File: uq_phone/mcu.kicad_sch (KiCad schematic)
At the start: 22 parts, among them J5 FTSH-105-XX-X-DV, J6 Conn_ARM_SWD_TagConnect_TC2030, U5 TXB0108RGYR, U6 TXB0108RGYR, U7 STM32H730VBTx

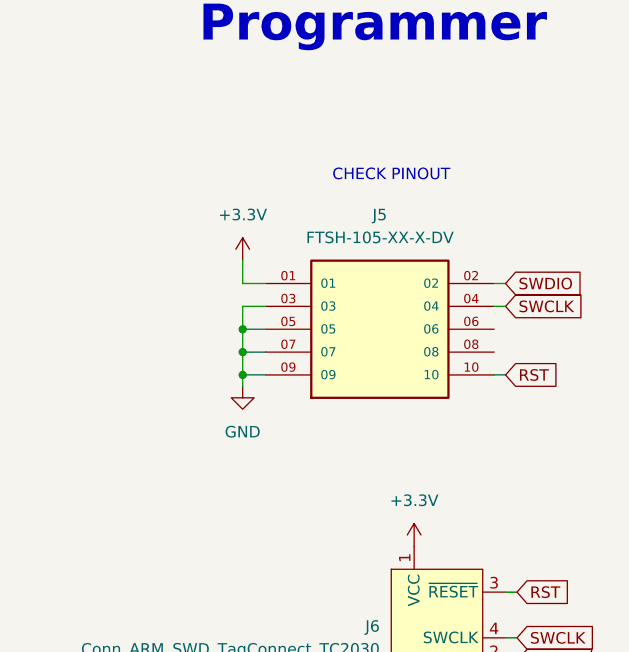
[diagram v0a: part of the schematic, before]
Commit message: Update routing
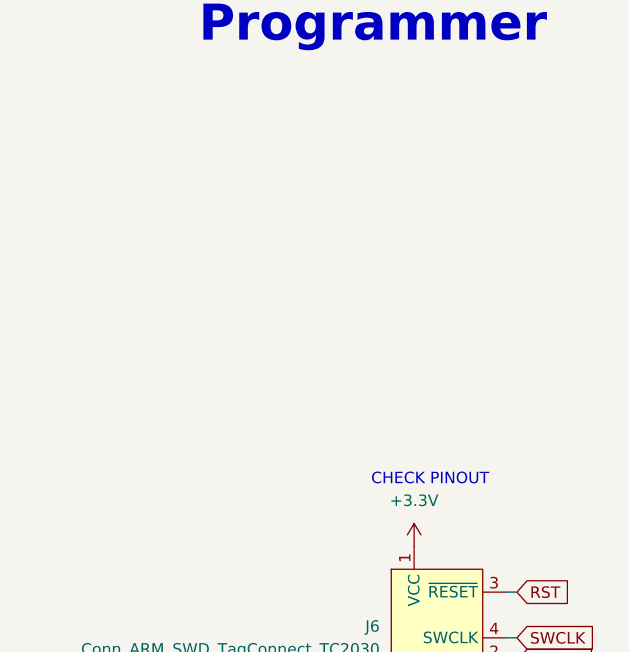
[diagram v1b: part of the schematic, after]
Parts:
- removed J5: FTSH-105-XX-X-DV, FTSH-105-XX-X-DV:SAMTEC_FTSH-105-XX-X-DV, symbol FTSH-105-XX-X-DV:FTSH-105-XX-X-DV
